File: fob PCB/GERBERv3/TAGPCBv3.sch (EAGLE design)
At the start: 8 parts, among them IC1 DWM1000

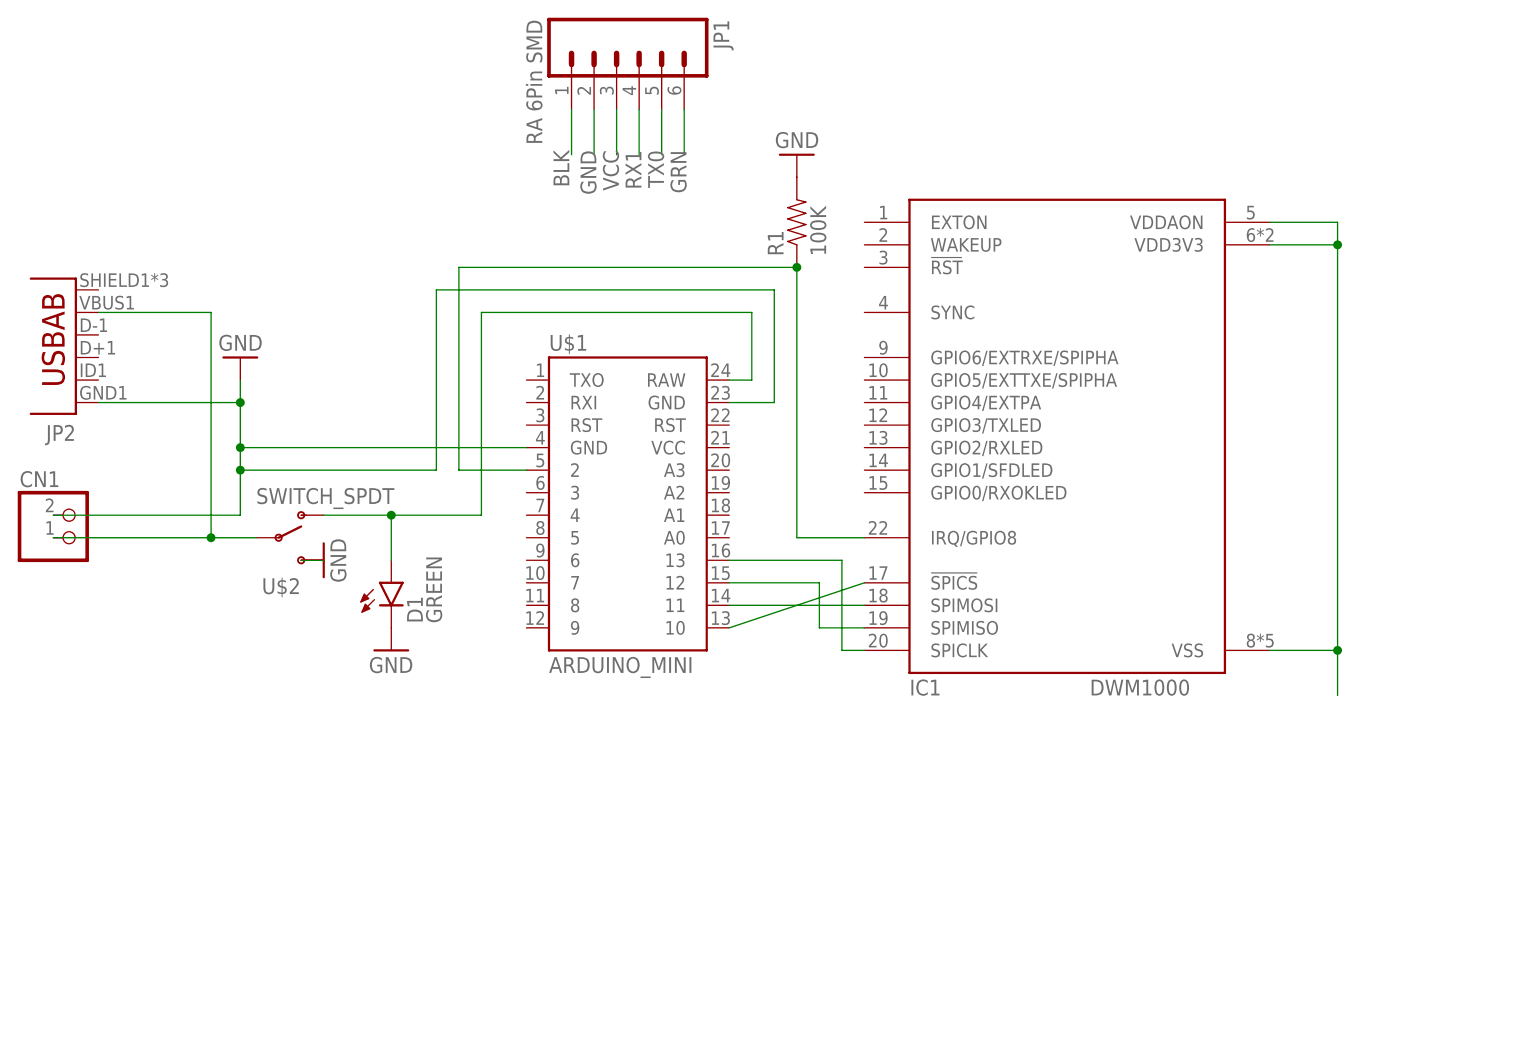
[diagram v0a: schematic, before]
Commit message: fob PCB Updated
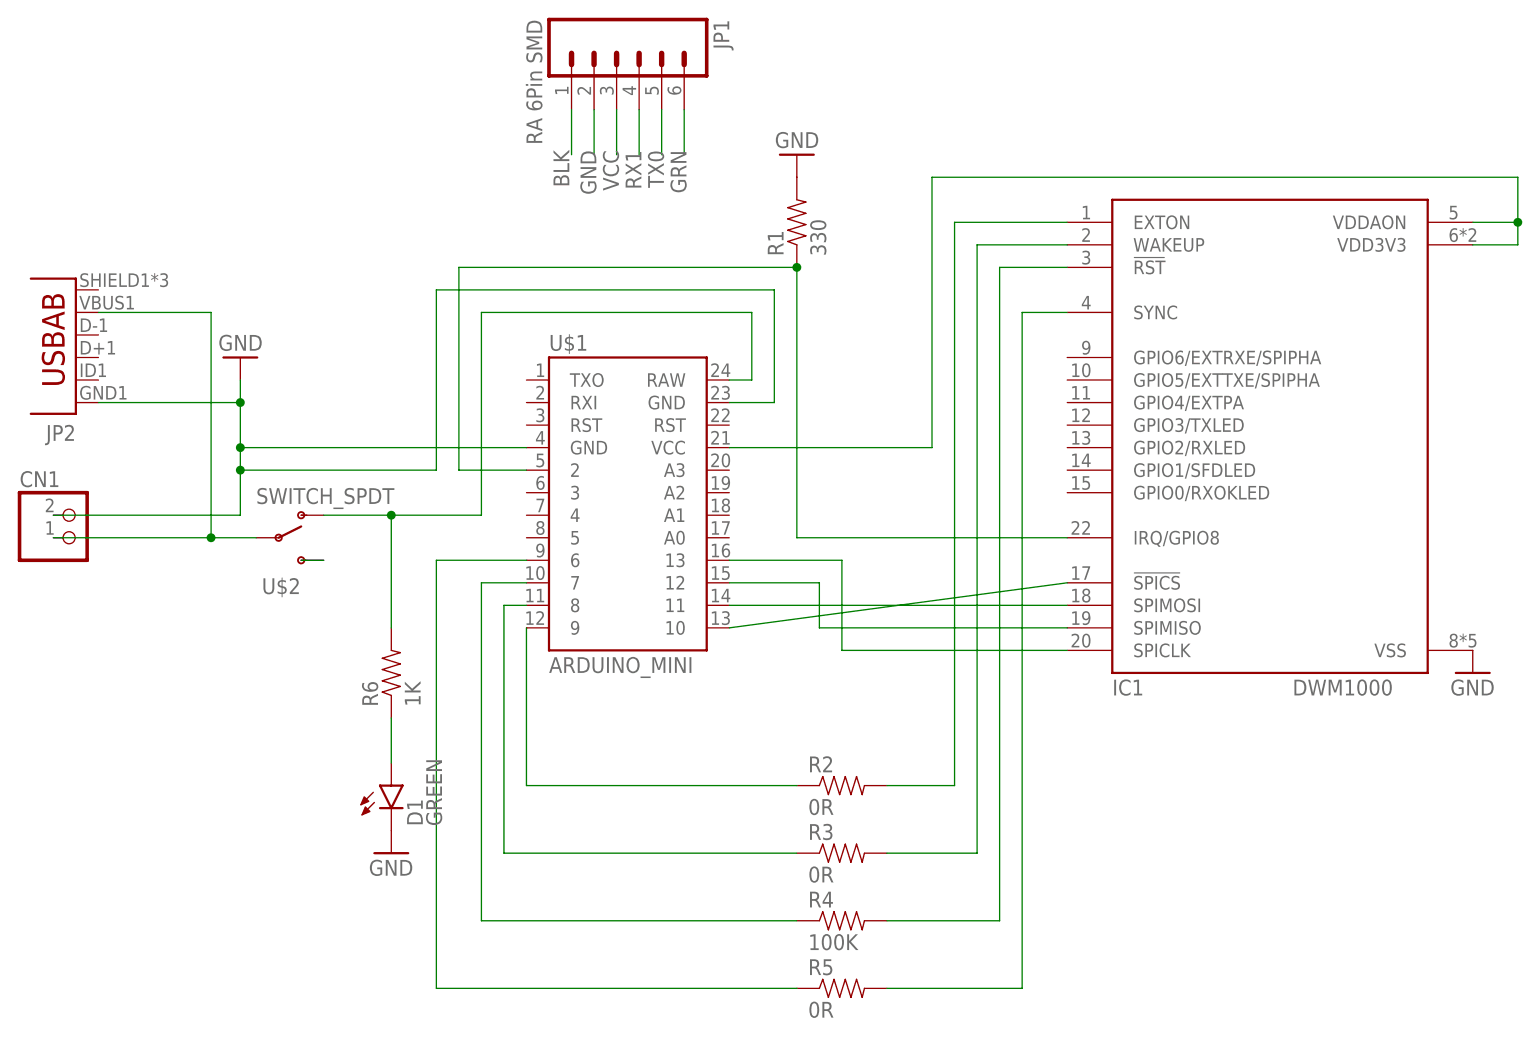
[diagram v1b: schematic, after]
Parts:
- added R2, R3, R5: 0R, SparkFun-Resistors:RESISTOR1206
- added R4: 100K, SparkFun-Resistors:RESISTOR1206
- added R6: 1K, SparkFun-Resistors:RESISTOR1206
- R1: value 100K -> 330
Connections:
- new net N$10: IC1.EXTON, R2.2
- new net N$11: R3.1, U$1.8
- new net N$12: IC1.WAKEUP, R3.2
- new net N$13: IC1.!RST, R4.2
- new net N$14: R4.1, U$1.7
- new net N$15: R5.1, U$1.6
- new net N$16: IC1.SYNC, R5.2
- new net N$17: U$2.S
- new net N$18: D1.A, R6.1
- new net N$9: R2.1, U$1.9
- net GND: now also IC1.VSS; no longer U$2.S
- net N$6: now also R6.2; no longer D1.A
- net N$8: now also U$1.VCC; no longer IC1.VSS
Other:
- moved on the sheet: D1, IC1
